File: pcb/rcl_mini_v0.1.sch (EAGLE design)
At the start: 60 parts, among them CN1 USB mini B, Q1 8MHz, Q2 IRLML5203, U1 MCP6002T-I/SN, U2 MCP6002T-I/SN, U3 MCP6002T-I/SN, U4 STM32F100CBT6, U5 MCP73831/OT, U6 MCP1703CB, X1 BAT, X2 TWEEZERS, X3 OLED, X4 SWD

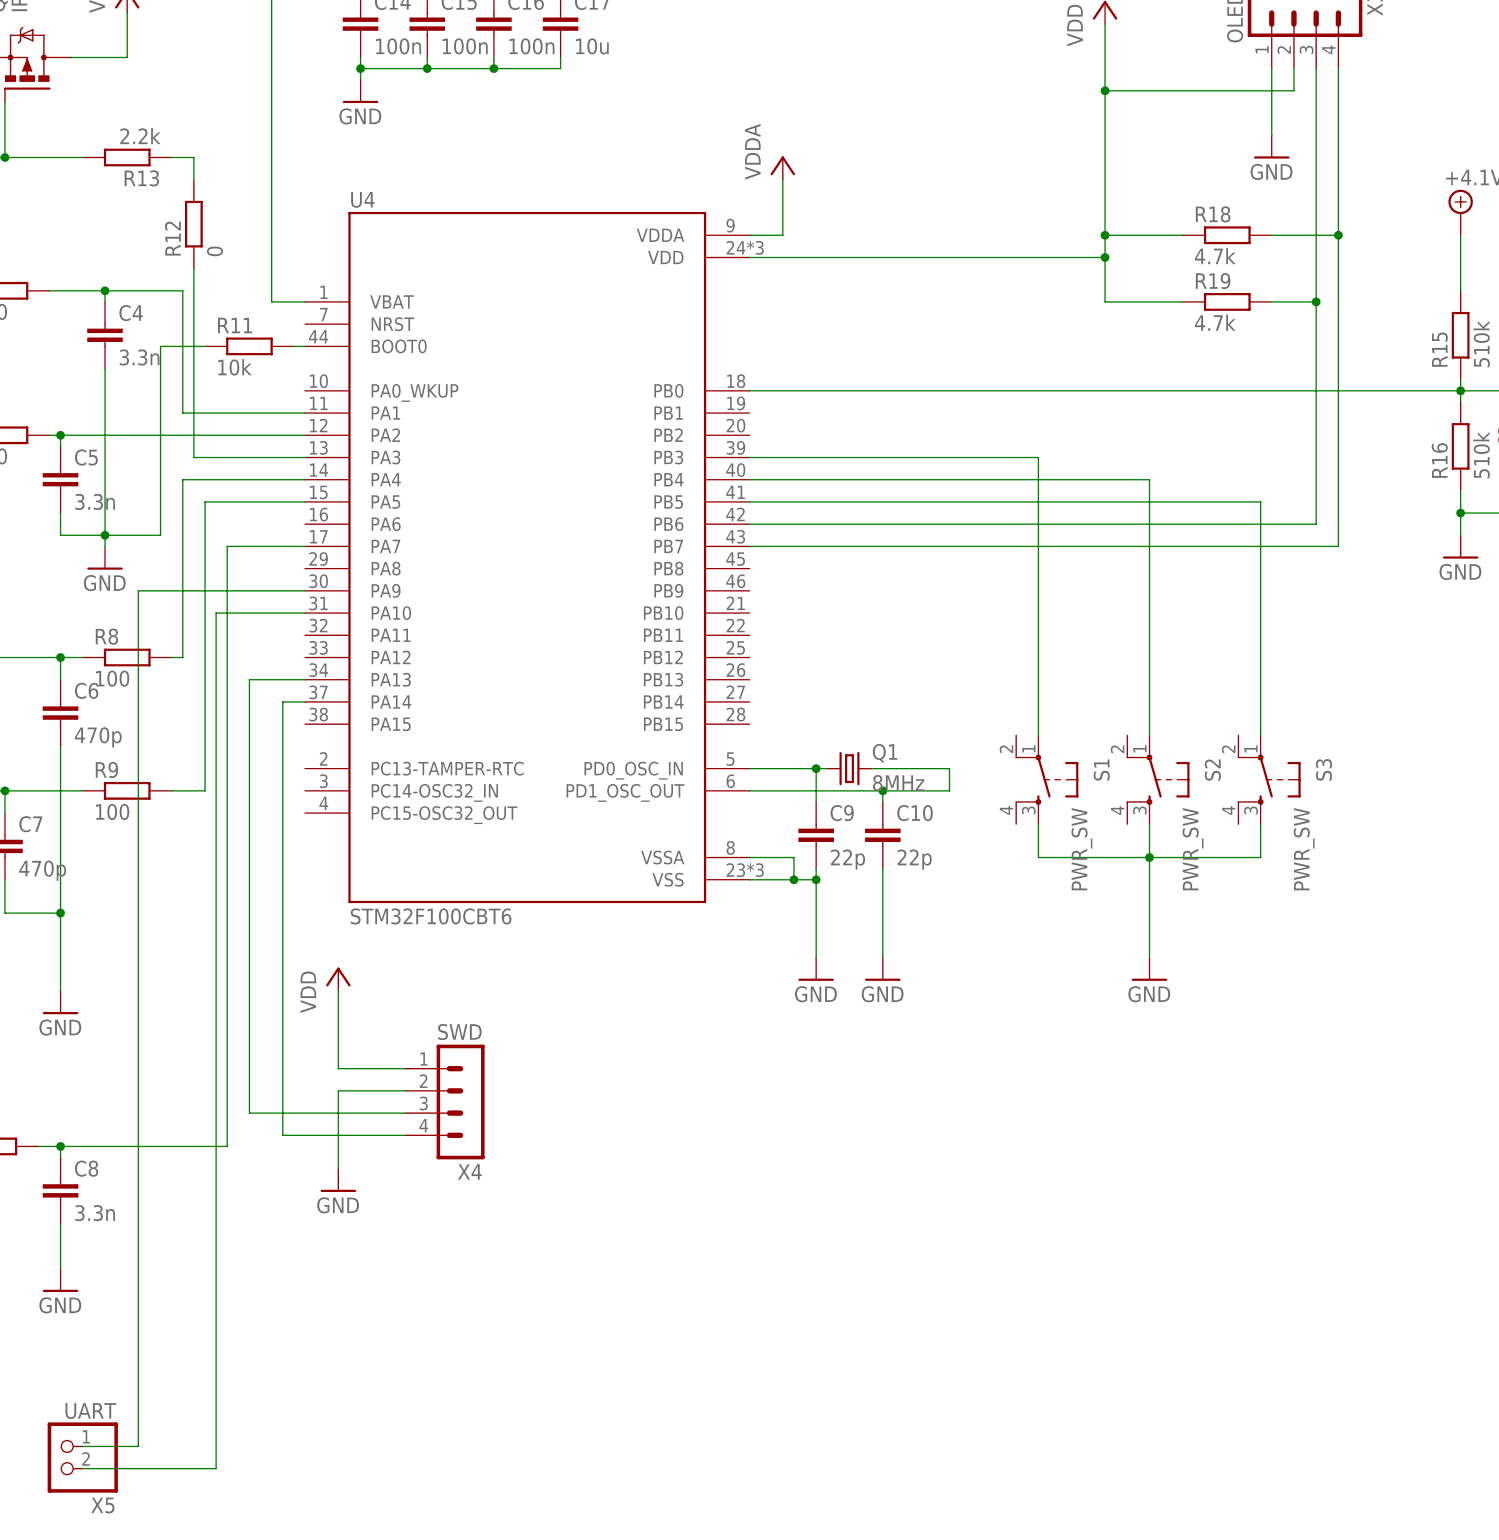
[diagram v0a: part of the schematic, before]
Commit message: pcb v1.0
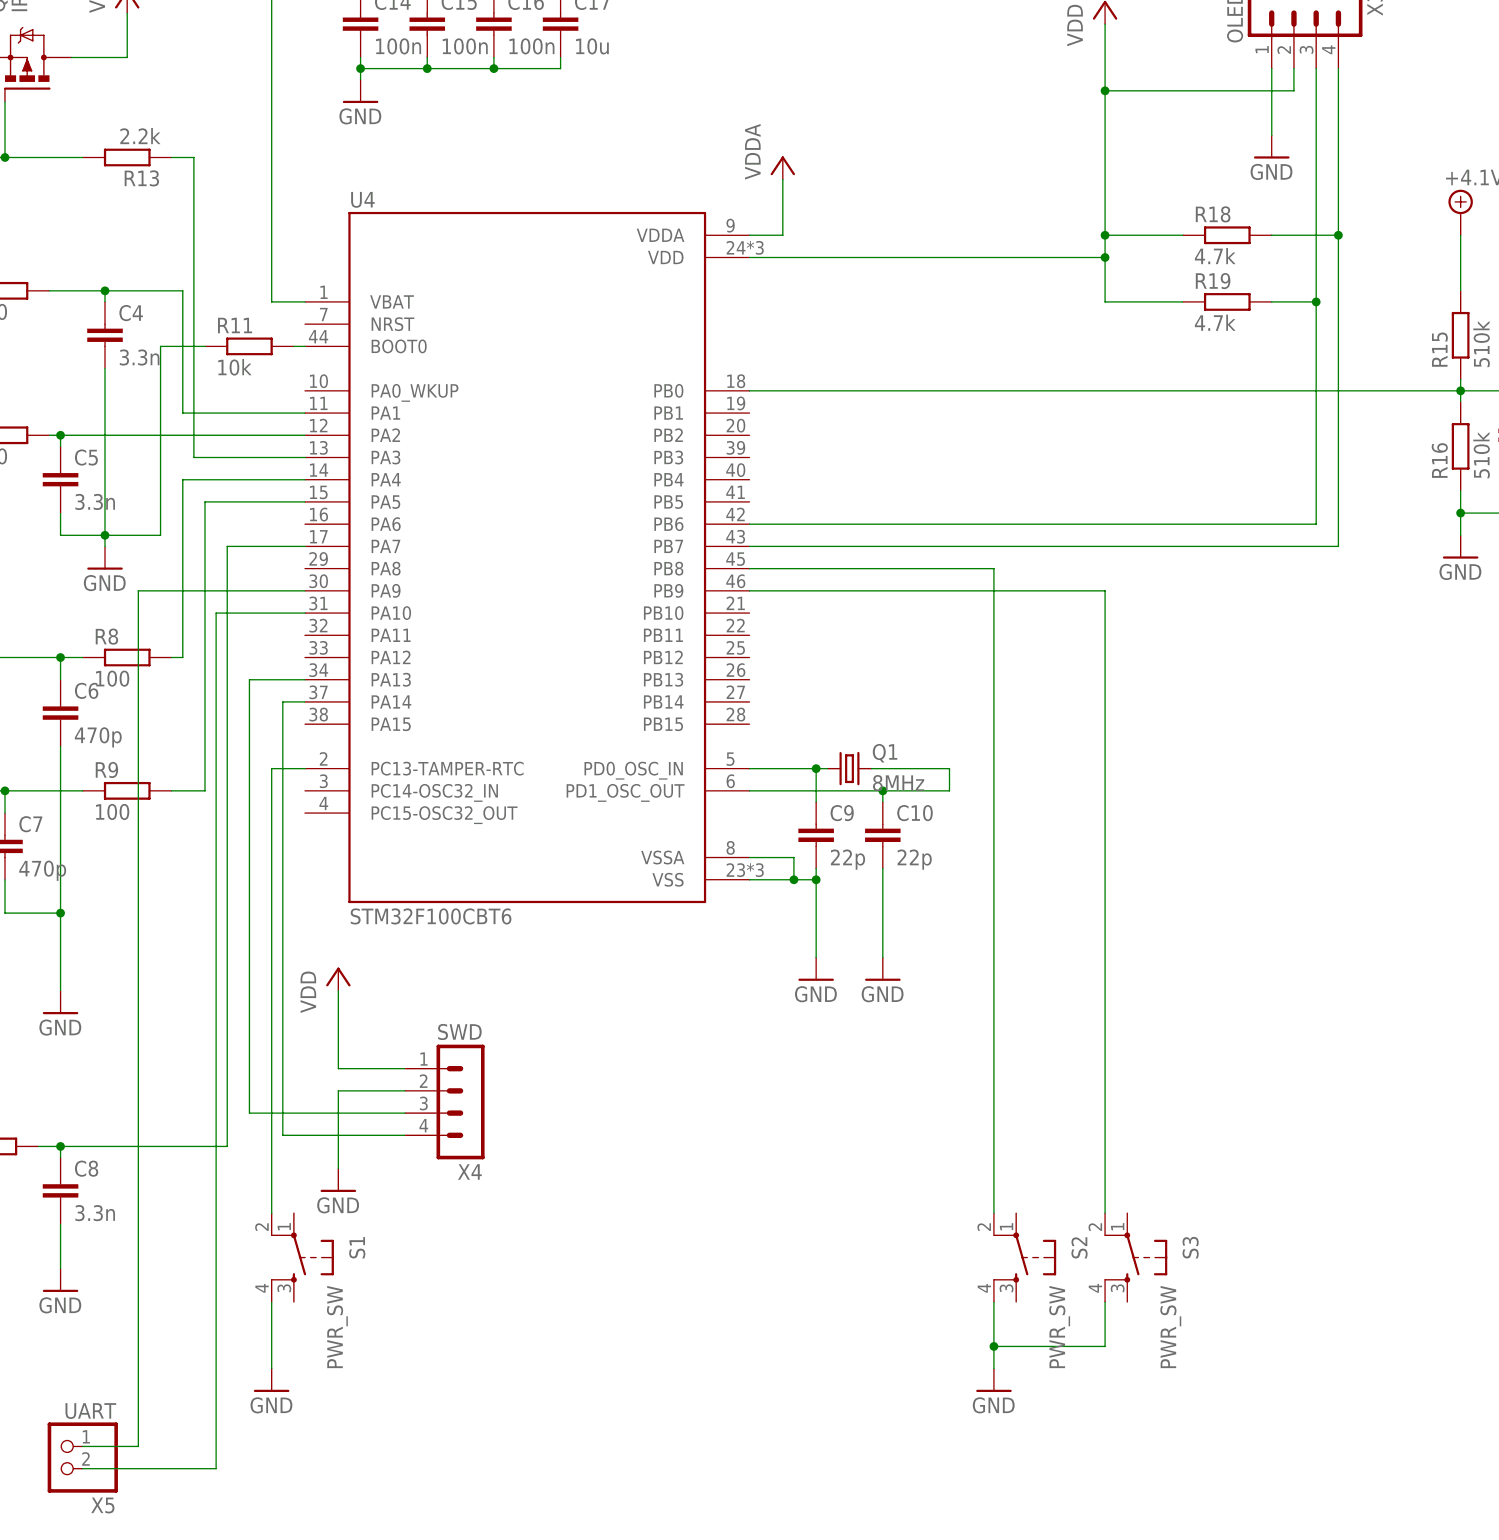
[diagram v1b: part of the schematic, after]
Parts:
- removed R12: 0, rcl:R-EU_R1206
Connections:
- removed net N$1: R12.2, R13.1
- net GND: now also S1.4, S2.4, S3.4; no longer S1.3, S2.3, S3.3
- net PA3: now also R13.1; no longer R12.1
- net SW1: now also S1.2, U4.PC13-TAMPER-RTC; no longer S1.1, U4.PB3
- net SW2: now also S2.2, U4.PB8; no longer S2.1, U4.PB4
- net SW3: now also S3.2, U4.PB9; no longer S3.1, U4.PB5
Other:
- moved on the sheet: S1, S2, S3
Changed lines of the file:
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@@
 <part name="GND11" library="supply1" deviceset="GND" device=""/>
 <part name="S1" library="switch-tact" deviceset="DTS-6" device="" value="PWR_SW"/>
+<part name="GND12" library="supply1" deviceset="GND" device=""/>
 <part name="S2" library="switch-tact" deviceset="DTS-6" device="" value="PWR_SW"/>
 <part name="GND13" library="supply1" deviceset="GND" device=""/>
@@
 <part name="R18" library="rcl" deviceset="R-EU_" device="M0805" value="4.7k"/>
 <part name="R19" library="rcl" deviceset="R-EU_" device="M0805" value="4.7k"/>
-<part name="R12" library="rcl" deviceset="R-EU_" device="R1206" value="0"/>
 </parts>
 <sheets>
@@
 <instance part="GND10" gate="1" x="128.27" y="102.87"/>
 <instance part="GND11" gate="1" x="135.89" y="102.87"/>
-<instance part="S1" gate="G$1" x="153.67" y="125.73" rot="R180"/>
-<instance part="S2" gate="G$1" x="166.37" y="125.73" rot="R180"/>
-<instance part="GND13" gate="1" x="166.37" y="102.87"/>
-<instance part="S3" gate="G$1" x="179.07" y="125.73" rot="R180"/>
+<instance part="S1" gate="G$1" x="68.58" y="71.12" rot="R180"/>
+<instance part="GND12" gate="1" x="66.04" y="55.88"/>
+<instance part="S2" gate="G$1" x="151.13" y="71.12" rot="R180"/>
+<instance part="GND13" gate="1" x="148.59" y="55.88"/>
+<instance part="S3" gate="G$1" x="163.83" y="71.12" rot="R180"/>
 <instance part="X3" gate="1" x="185.42" y="214.63" rot="R270"/>
 <instance part="GND14" gate="1" x="180.34" y="196.85"/>
@@
 <instance part="R18" gate="G$1" x="175.26" y="187.96"/>
 <instance part="R19" gate="G$1" x="175.26" y="180.34"/>
-<instance part="R12" gate="G$1" x="57.15" y="189.23" rot="R90"/>
 </instances>
 <busses>
@@
 <pinref part="GND11" gate="1" pin="GND"/>
 <wire x1="135.89" y1="115.57" x2="135.89" y2="105.41" width="0.1524" layer="91"/>
+</segment>
+<segment>
+<pinref part="S1" gate="G$1" pin="4"/>
+<pinref part="GND12" gate="1" pin="GND"/>
+<wire x1="66.04" y1="66.04" x2="66.04" y2="58.42" width="0.1524" layer="91"/>
+</segment>
+<segment>
+<pinref part="S2" gate="G$1" pin="4"/>
+<pinref part="GND13" gate="1" pin="GND"/>
+<wire x1="148.59" y1="66.04" x2="148.59" y2="60.96" width="0.1524" layer="91"/>
+<pinref part="S3" gate="G$1" pin="4"/>
+<wire x1="148.59" y1="60.96" x2="148.59" y2="58.42" width="0.1524" layer="91"/>
+<wire x1="161.29" y1="66.04" x2="161.29" y2="60.96" width="0.1524" layer="91"/>
+<wire x1="161.29" y1="60.96" x2="148.59" y2="60.96" width="0.1524" layer="91"/>
+<junction x="148.59" y="60.96"/>
 </segment>
 <segment>
@@
 <junction x="-44.45" y="204.47"/>
 </segment>
-<segment>
-<pinref part="S2" gate="G$1" pin="3"/>
-<pinref part="GND13" gate="1" pin="GND"/>
-<wire x1="166.37" y1="120.65" x2="166.37" y2="116.84" width="0.1524" layer="91"/>
-<pinref part="S1" gate="G$1" pin="3"/>
-<wire x1="166.37" y1="116.84" x2="166.37" y2="105.41" width="0.1524" layer="91"/>
-<wire x1="153.67" y1="120.65" x2="153.67" y2="116.84" width="0.1524" layer="91"/>
-<wire x1="153.67" y1="116.84" x2="166.37" y2="116.84" width="0.1524" layer="91"/>
-<junction x="166.37" y="116.84"/>
-<pinref part="S3" gate="G$1" pin="3"/>
-<wire x1="179.07" y1="120.65" x2="179.07" y2="116.84" width="0.1524" layer="91"/>
-<wire x1="179.07" y1="116.84" x2="166.37" y2="116.84" width="0.1524" layer="91"/>
-</segment>
 </net>
 <net name="USB+" class="0">
@@
 </segment>
 </net>
+<net name="SW1" class="0">
+<segment>
+<pinref part="S1" gate="G$1" pin="2"/>
+<wire x1="66.04" y1="76.2" x2="66.04" y2="127" width="0.1524" layer="91"/>
+<pinref part="U4" gate="G$1" pin="PC13-TAMPER-RTC"/>
+<wire x1="66.04" y1="127" x2="69.85" y2="127" width="0.1524" layer="91"/>
+</segment>
+</net>
+<net name="SW2" class="0">
+<segment>
+<pinref part="U4" gate="G$1" pin="PB8"/>
+<pinref part="S2" gate="G$1" pin="2"/>
+<wire x1="120.65" y1="149.86" x2="148.59" y2="149.86" width="0.1524" layer="91"/>
+<wire x1="148.59" y1="149.86" x2="148.59" y2="76.2" width="0.1524" layer="91"/>
+</segment>
+</net>
+<net name="SW3" class="0">
+<segment>
+<pinref part="U4" gate="G$1" pin="PB9"/>
+<pinref part="S3" gate="G$1" pin="2"/>
+<wire x1="120.65" y1="147.32" x2="161.29" y2="147.32" width="0.1524" layer="91"/>
+<wire x1="161.29" y1="147.32" x2="161.29" y2="76.2" width="0.1524" layer="91"/>
+</segment>
+</net>
 <net name="OLED_I2C_SCK" class="0">
 <segment>
@@
 <pinref part="U4" gate="G$1" pin="PA3"/>
 <wire x1="69.85" y1="162.56" x2="57.15" y2="162.56" width="0.1524" layer="91"/>
-<pinref part="R12" gate="G$1" pin="1"/>
-<wire x1="57.15" y1="184.15" x2="57.15" y2="162.56" width="0.1524" layer="91"/>
+<wire x1="57.15" y1="162.56" x2="57.15" y2="196.85" width="0.1524" layer="91"/>
+<pinref part="R13" gate="G$1" pin="1"/>
+<wire x1="57.15" y1="196.85" x2="54.61" y2="196.85" width="0.1524" layer="91"/>
 </segment>
 </net>
@@
 </segment>
 </net>
-<net name="SW1" class="0">
-<segment>
-<pinref part="U4" gate="G$1" pin="PB3"/>
-<pinref part="S1" gate="G$1" pin="1"/>
-<wire x1="120.65" y1="162.56" x2="153.67" y2="162.56" width="0.1524" layer="91"/>
-<wire x1="153.67" y1="162.56" x2="153.67" y2="130.81" width="0.1524" layer="91"/>
-</segment>
-</net>
-<net name="SW2" class="0">
-<segment>
-<pinref part="U4" gate="G$1" pin="PB4"/>
-<pinref part="S2" gate="G$1" pin="1"/>
-<wire x1="120.65" y1="160.02" x2="166.37" y2="160.02" width="0.1524" layer="91"/>
-<wire x1="166.37" y1="160.02" x2="166.37" y2="130.81" width="0.1524" layer="91"/>
-</segment>
-</net>
-<net name="SW3" class="0">
-<segment>
-<pinref part="U4" gate="G$1" pin="PB5"/>
-<pinref part="S3" gate="G$1" pin="1"/>
-<wire x1="120.65" y1="157.48" x2="179.07" y2="157.48" width="0.1524" layer="91"/>
-<wire x1="179.07" y1="157.48" x2="179.07" y2="130.81" width="0.1524" layer="91"/>
-</segment>
-</net>
-<net name="N$1" class="0">
-<segment>
-<pinref part="R13" gate="G$1" pin="1"/>
-<wire x1="57.15" y1="196.85" x2="54.61" y2="196.85" width="0.1524" layer="91"/>
-<pinref part="R12" gate="G$1" pin="2"/>
-<wire x1="57.15" y1="196.85" x2="57.15" y2="194.31" width="0.1524" layer="91"/>
-</segment>
-</net>
